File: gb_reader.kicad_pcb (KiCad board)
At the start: 2 copper layers, 120 x 87.5 mm, 46 parts, among them J1 USB_B_Micro, J2 Conn_01x09, J3 Conn_01x04, J4 Conn_01x32, J5 Conn_01x32_MountingPin, SW1 SW_Push, SW2 SW_Push, SW3 SW_Push, SW4 SW_Push, U1 STM32F103RFTx, U2 TLV70233_SOT23-5, U3 TXB0108PWR, U4 TXB0108PWR, U5 TXB0108PWR, U6 TXB0108PWR, Y1 32kHz

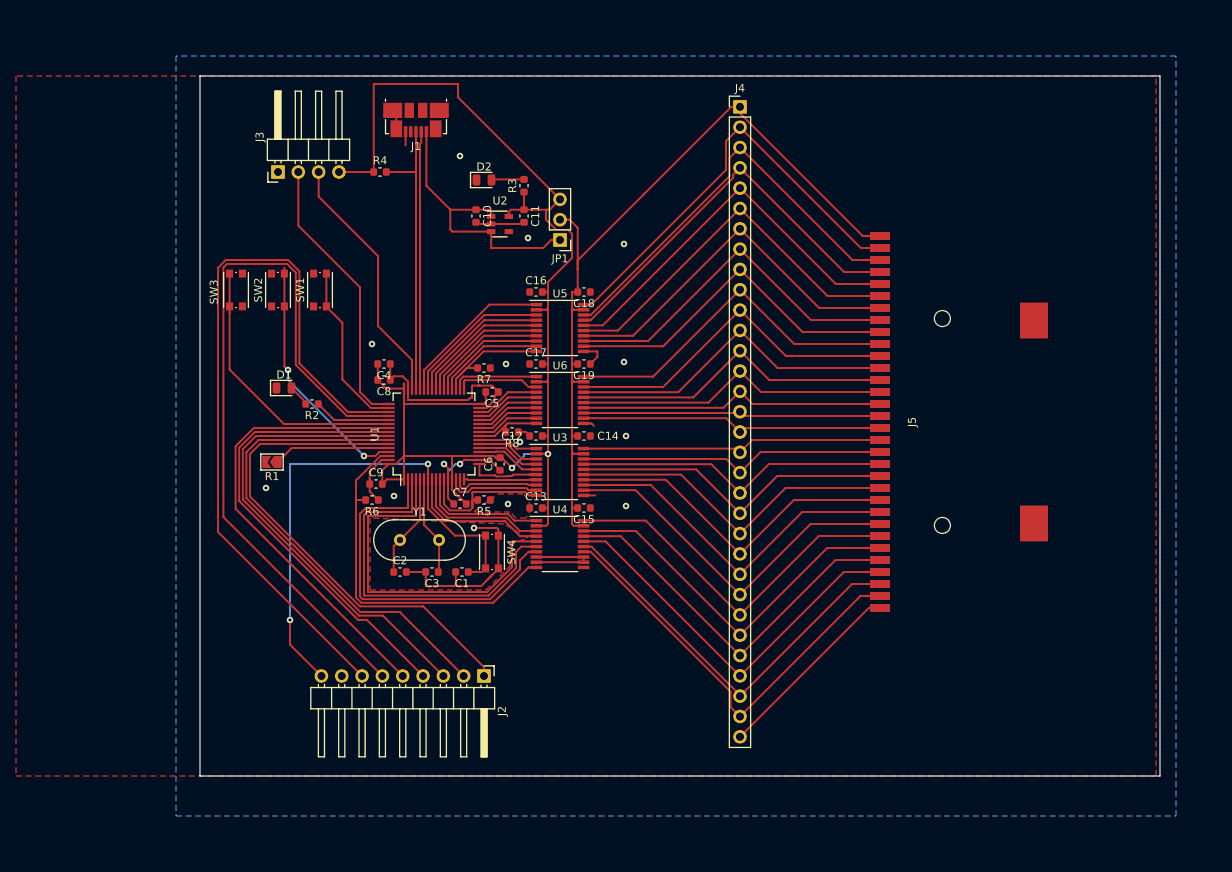
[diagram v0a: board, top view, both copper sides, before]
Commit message: Done
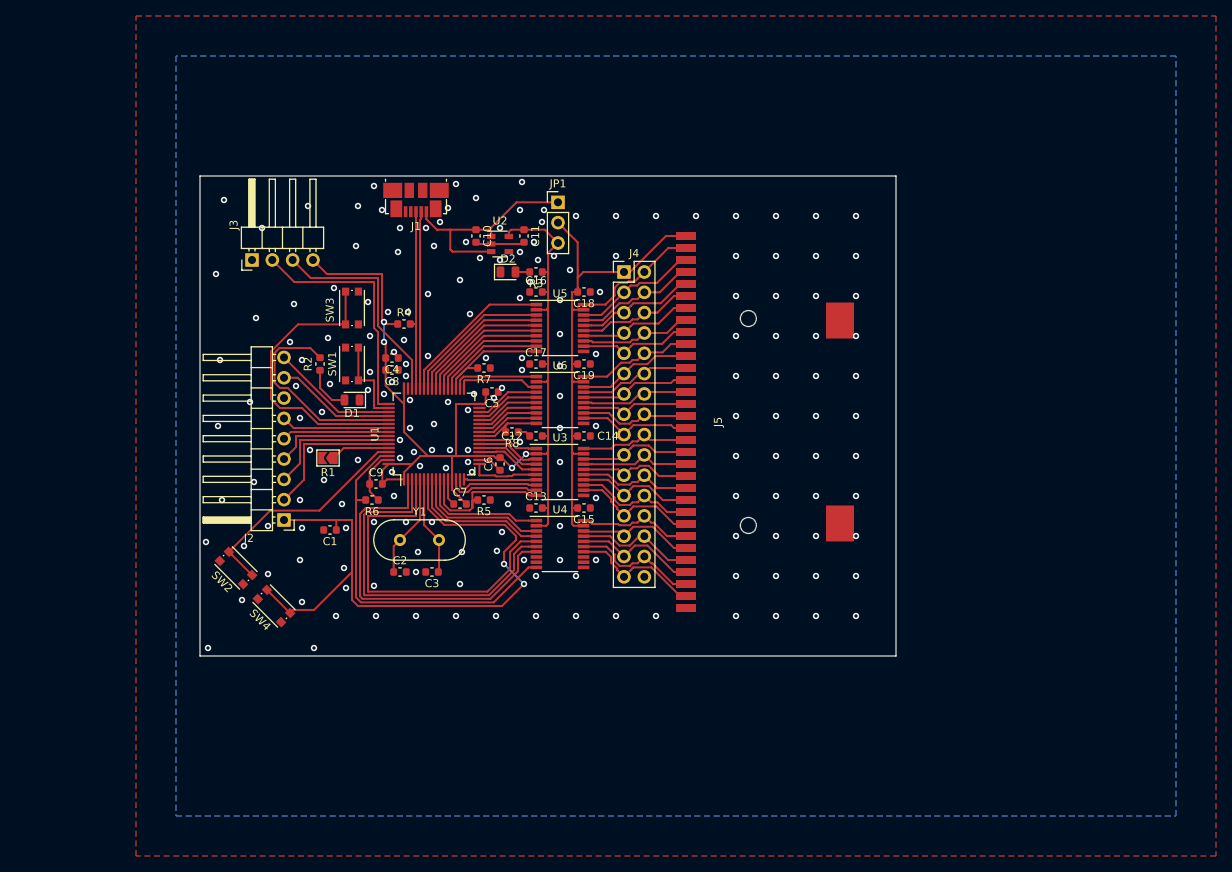
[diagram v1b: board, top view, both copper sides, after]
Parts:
- J4: footprint Connector_PinHeader_2.54mm:PinHeader_1x32_P2.54mm_Vertical -> Connector_PinHeader_2.54mm:PinHeader_2x16_P2.54mm_Vertical
- moved SW2 35.1 mm to (112.5, 104.0), turned to 135 degrees
- moved J2 31.7 mm to (118.5, 98.0), turned to 180 degrees
- moved SW4 28.1 mm to (117.2, 108.8), turned to 135 degrees
- moved J4 25.2 mm to (161.0, 67.0)
- moved J5 24.2 mm to (174.5, 85.8)
- moved R4 19.2 mm to (133.5, 73.5)
- moved C1 17.3 mm to (124.2, 99.2)
- moved SW3 14.7 mm to (127.0, 71.5)
- moved D2 11.9 mm to (146.5, 67.0)
- moved J3 11.5 mm to (114.5, 65.5)
- moved R3 10.9 mm to (150.0, 67.0), turned to 180 degrees
- moved SW1 10.1 mm to (127.0, 78.5)
- moved J1 10.0 mm to (135.0, 58.0)
- moved D1 8.63 mm to (127.0, 83.0), turned to 180 degrees
- moved R1 7.02 mm to (124.0, 90.2)
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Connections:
- J1 pad 4: (no net) -> Net-(J1-Pad4)
- J2 pad 1: I2C_SDA -> /NRST
- J2 pad 2: I2C_SCL -> I2C_SDA
- J2 pad 3: SPI_MOSI -> I2C_SCL
- J2 pad 4: SPI_MISO -> SPI_MOSI
- J2 pad 5: SPI_SCK -> SPI_MISO
- J2 pad 6: UART4_RX -> SPI_SCK
- J2 pad 7: UART4_TX -> Net-(J2-Pad7)
- J2 pad 8: (no net) -> UART4_RX
- J2 pad 9: /NRST -> UART4_TX
- U2 pad 4: (no net) -> Net-(U2-Pad4)
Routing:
- net GND: track 124.5 -> 21.2 mm, vias 15 -> 190
- net UART4_RX: track 94.7 -> 15.1 mm
- net UART4_TX: track 94.8 -> 15.9 mm
- net SPI_MISO: track 58.2 -> 13.4 mm
- net SPI_MOSI: track 59.4 -> 15.1 mm
- net SPI_SCK: track 57.7 -> 13.6 mm
- net I2C_SCL: track 60.7 -> 16.8 mm
- net I2C_SDA: track 62.4 -> 18.6 mm
- net Pak-Vcc: track 102.9 -> 63.4 mm
- net CAR_CLK: track 54.6 -> 16.3 mm
- net CAR_WR: track 52.9 -> 15.6 mm
- net CAR_ADI: track 52.9 -> 16.6 mm
- net CAR_RD: track 50.6 -> 15.3 mm
- net CAR_RST: track 50.7 -> 16.2 mm
- net CAR_CS: track 49.1 -> 14.9 mm
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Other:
- board size 120 x 87.5 mm -> 87 x 60 mm
